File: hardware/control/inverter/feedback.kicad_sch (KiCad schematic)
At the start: 20 parts, among them J7 PINHD_1x2_Male, J8 PINHD_1x2_Male, U15 TL3116

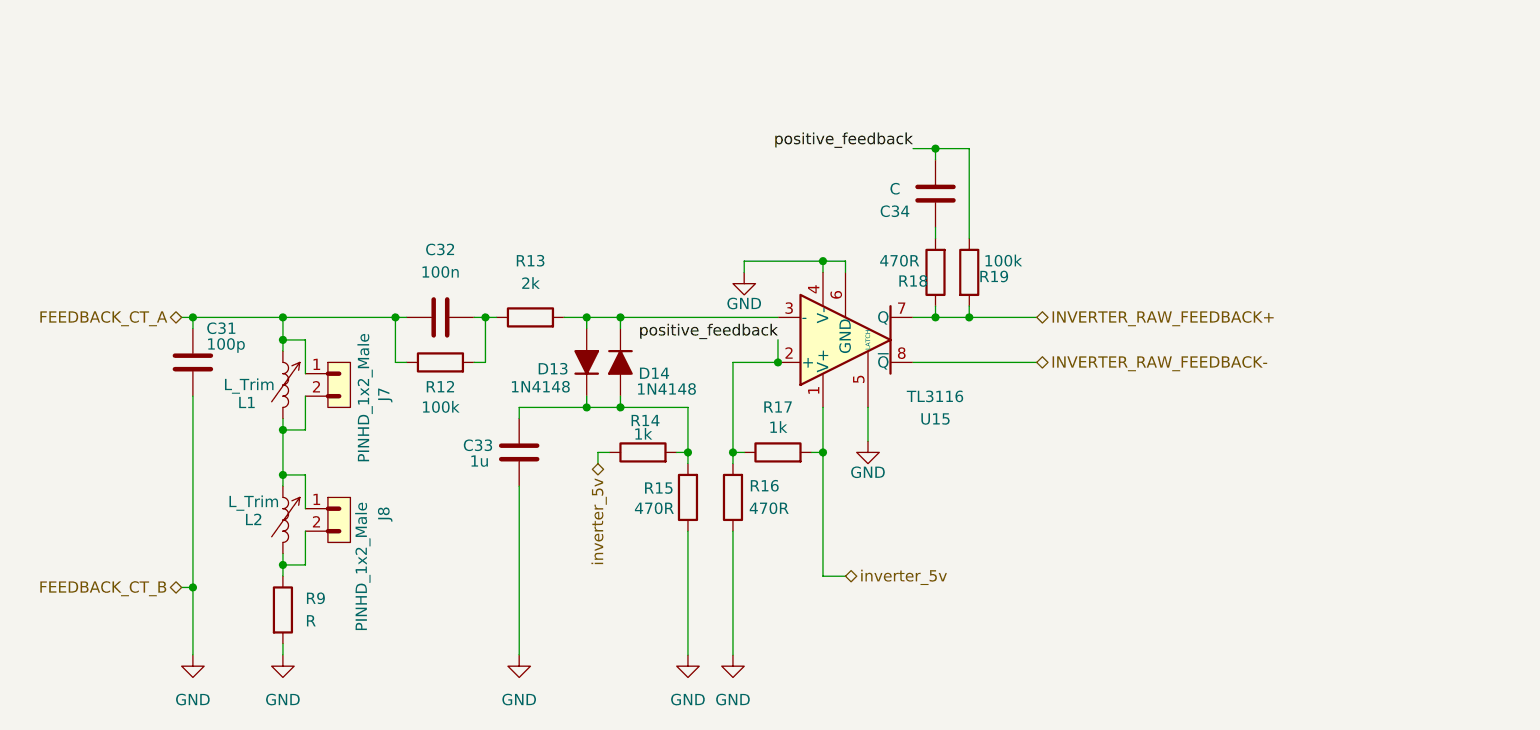
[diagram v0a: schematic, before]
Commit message: update right about freaking everything
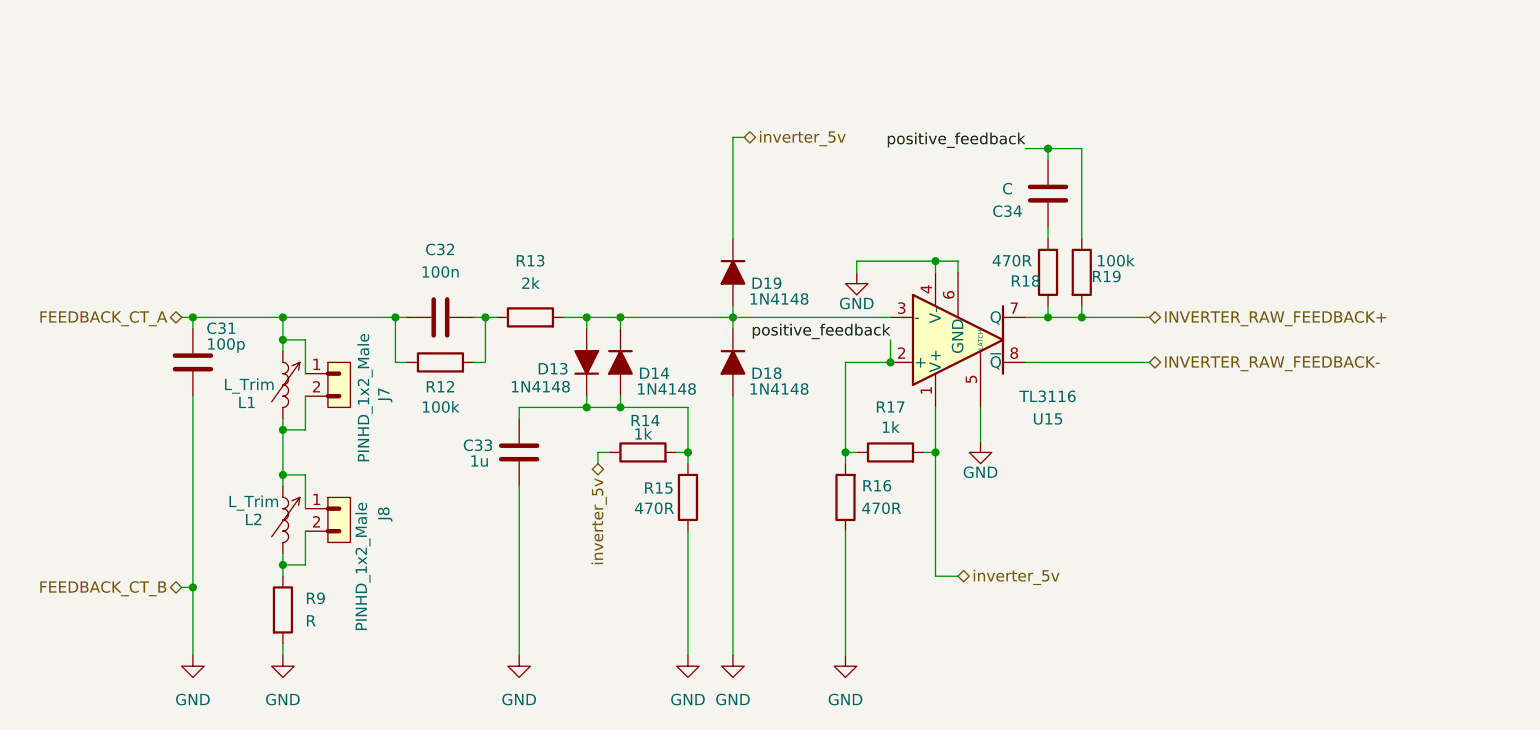
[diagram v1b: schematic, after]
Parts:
- added D18, D19: 1N4148, PCM_Diode_THT_AKL:D_DO-35_SOD27_P7.62mm_Horizontal, symbol PCM_Diode_AKL:1N4148
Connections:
- net GND: now also D18.2 (A)
- net inverter_5v: now also D19.1 (K)
- net at D13.2 (A), D14.1 (K), R13.2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: now also D18.1 (K), D19.2 (A)
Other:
- moved on the sheet: C34, R16, R17, R18, R19, U15

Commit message: idk some changes
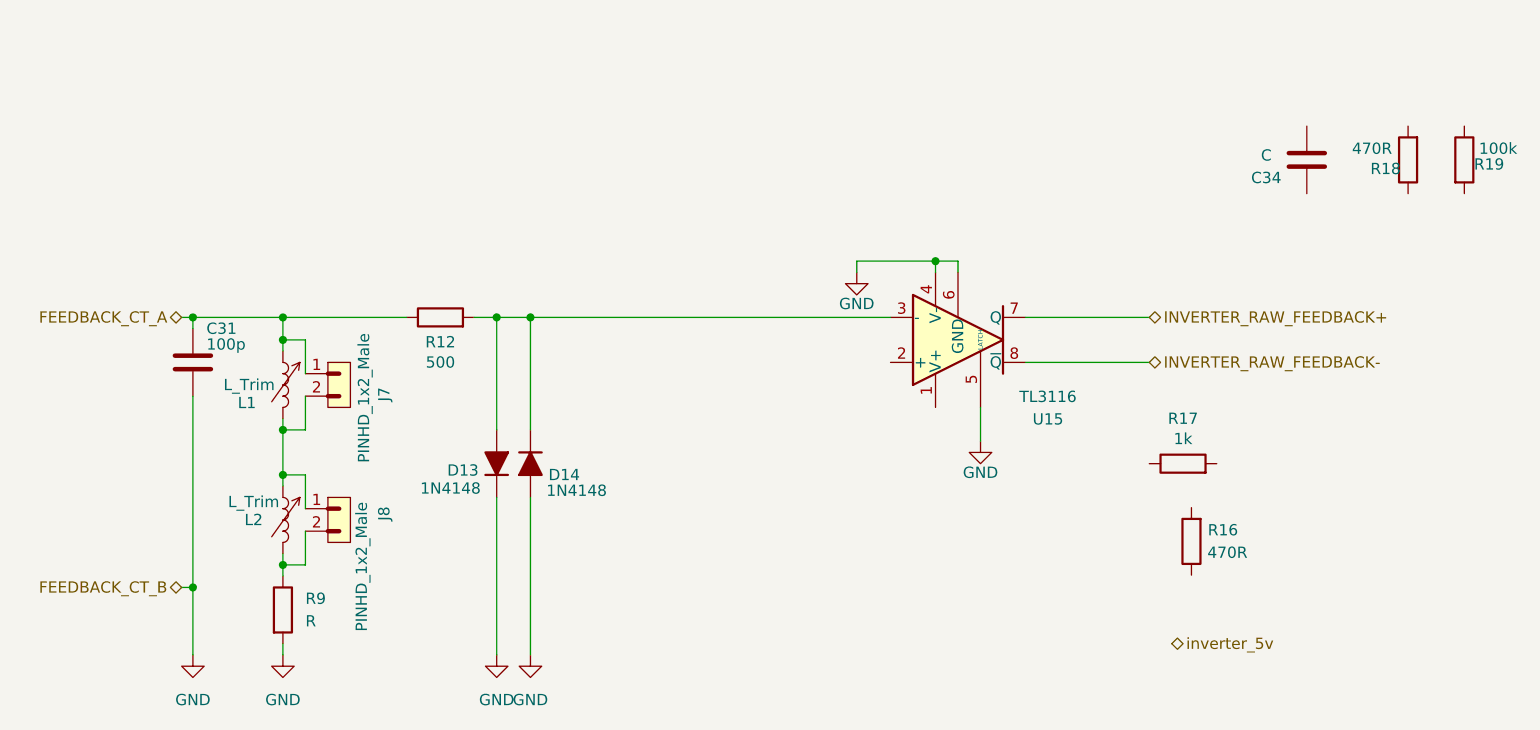
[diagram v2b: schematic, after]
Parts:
- removed C32: 100n, symbol Device:C
- removed C33: 1u, symbol Device:C
- removed D18, D19: 1N4148, PCM_Diode_THT_AKL:D_DO-35_SOD27_P7.62mm_Horizontal, symbol PCM_Diode_AKL:1N4148
- removed R13: 2k, symbol Device:R
- removed R14: 1k, symbol Device:R
- removed R15: 470R, symbol Device:R
- R12: value 100k -> 500
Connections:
- net GND: now also D13.1 (K), D14.2 (A); no longer R16.1
- net INVERTER_RAW_FEEDBACK+: no longer R18.1, R19.2
- net inverter_5v: no longer R17.2, U15.1 (V+)
- net at R12.2: now also D13.2 (A), D14.1 (K), U15.3 (-)
- net at R18.2: no longer C34.1
- removed net positive_feedback: C34.2, R16.2, R17.1, R19.1, U15.2 (+)
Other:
- moved on the sheet: C34, D13, D14, R12, R16, R17, R18, R19

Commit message: completed-ish inverter board, probably not, but anyway
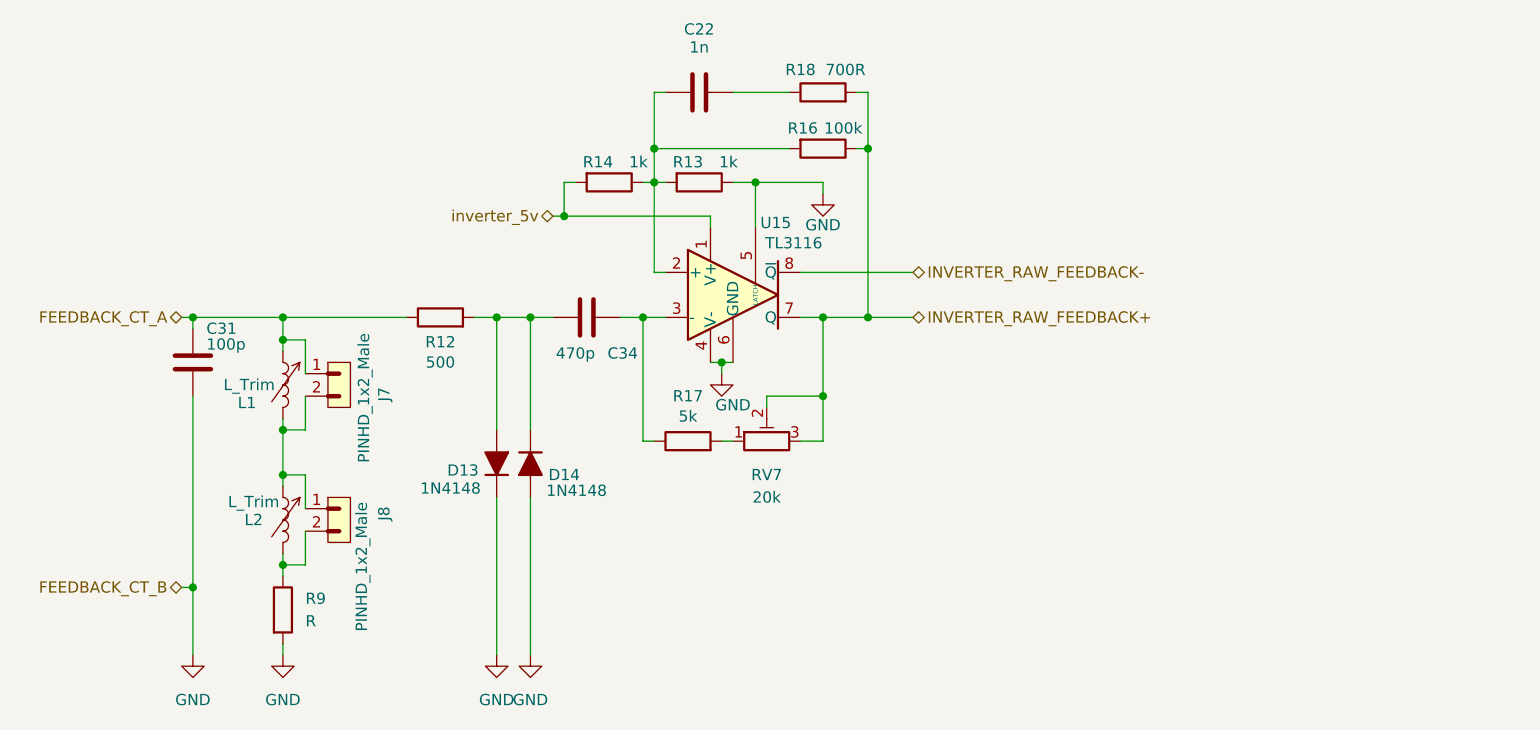
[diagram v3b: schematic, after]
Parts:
- removed R19: 100k, symbol Device:R
- added C22: 1n, symbol Device:C
- added R13, R14: 1k, symbol Device:R
- added RV7: 20k, symbol Device:R_Potentiometer_Trim
- C34: value C -> 470p
- R16: value 470R -> 100k
- R17: value 1k -> 5k
- R18: value 470R -> 700R
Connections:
- net GND: now also R13.1
- net INVERTER_RAW_FEEDBACK+: now also R16.1, R18.2, RV7.2, RV7.3
- net inverter_5v: now also U15.1 (V+), R14.2
- net at D13.2 (A), D14.1 (K), R12.2: now also C34.2; no longer U15.3 (-)
- net at R18.1: now also C22.2
- net at C34.1: now also R17.1, U15.3 (-)
- net at U15.2 (+): now also R16.2, C22.1, R13.2, R14.1
- net at R17.2: now also RV7.1
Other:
- moved on the sheet: C34, R16, R17, R18, U15
